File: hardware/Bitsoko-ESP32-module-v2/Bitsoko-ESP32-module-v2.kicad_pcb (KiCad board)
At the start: 2 copper layers, 40.6 x 27.9 mm, 4 parts, among them J1 CONN_02X10, J2 CONN_02X10, U1 ESP32-WROOM32-MODULE

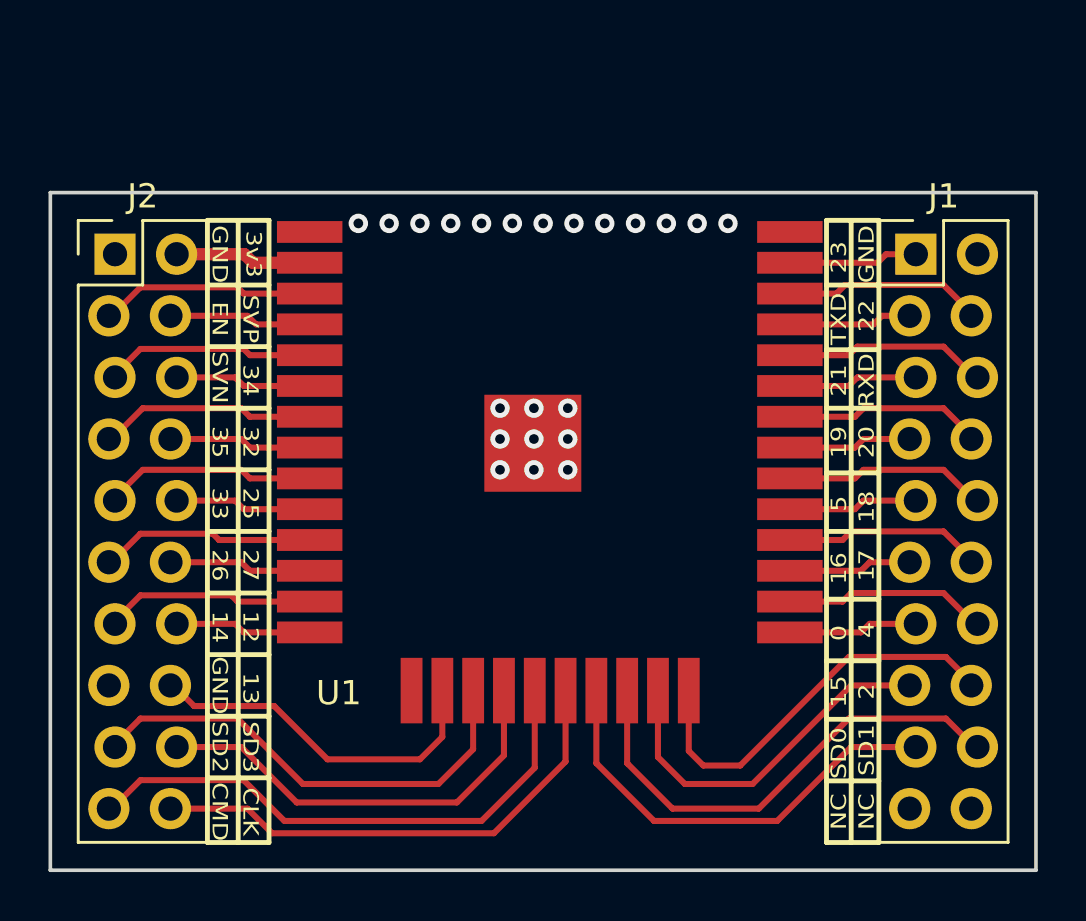
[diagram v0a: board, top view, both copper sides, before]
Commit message: Changed pin headers from a 5mil to 8 mil staggered offset for friction fitting in ESP32 module design.
This is due to testing on acrylic hat found the fitting not as solid for an electrical connection.
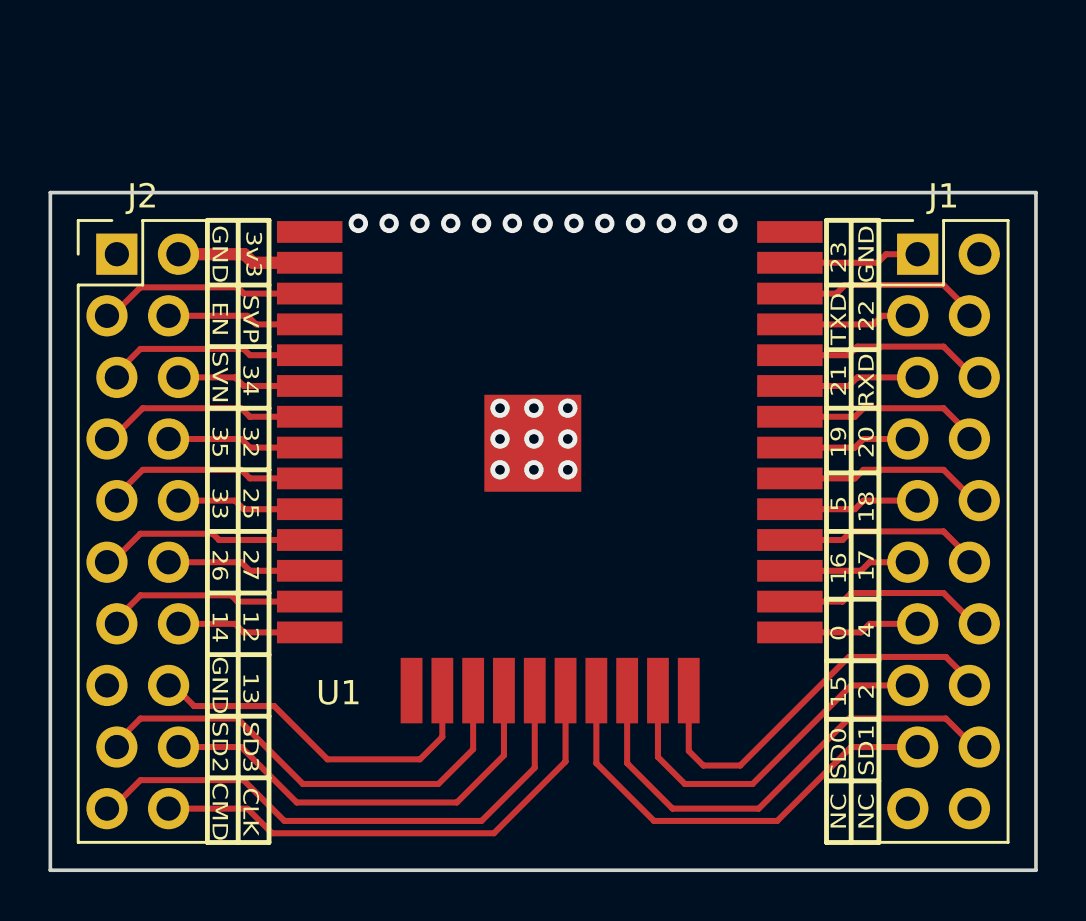
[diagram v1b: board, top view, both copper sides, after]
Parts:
- removed G***: LOGO, logos:bitsoko-logo
- J1, J2: footprint narra:Pin_Header_Straight_2x10_Pitch2.54mm_staggered -> narra:Pin_Header_Straight_2x10_Pitch2.54mm_8mil_staggered
